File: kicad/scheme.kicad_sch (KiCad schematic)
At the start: 46 parts, among them J1 reset, Q1 G1, SW1 SW_PUSH_6mm_H4.3mm, SW2 SW_PUSH_6mm_H4.3mm, SW3 SW_PUSH_6mm_H4.3mm, SW4 btn-start, SW5 SW_PUSH_6mm_H4.3mm, U1 COM-09032-103-530, U2 ESP-12E-no_pins, U3 PCA9306, U4 AP2112K-3.3, U5 ADS1015IDGS, U6 ME6211C18M5, U7 ICM-20948

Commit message: kicad-updates
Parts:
- removed ICM-conn1: AUX-ICM-no!, Connector_PinHeader_2.54mm:PinHeader_1x04_P2.54mm_Vertical, symbol Connector:Conn_01x04_Pin
- added J2: Conn_01x04, Connector_PinSocket_2.54mm:PinSocket_1x04_P2.54mm_Vertical, symbol Connector_Generic:Conn_01x04
- added J3: poweron, Connector_PinHeader_2.54mm:PinHeader_2x01_P2.54mm_Vertical, symbol Connector:Conn_01x02_Pin
- added R16: R-100, Resistor_SMD:R_0805_2012Metric, symbol models:R-10k
- added R17: 4k7, Resistor_SMD:R_0805_2012Metric_Pad1.20x1.40mm_HandSolder, symbol Device:R_Small
- added R18: 1k, Resistor_SMD:R_0805_2012Metric_Pad1.20x1.40mm_HandSolder, symbol Device:R_Small
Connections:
- net +3.3V: now also R16.2
- net +4.2V: now also J2.1 (Pin_1), J3.1 (Pin_1); no longer TP4056-module1.3 (out+)
- net GND: now also J2.2 (Pin_2), R18.2; no longer SW4.1 (C)
- net SCL: now also J2.3 (Pin_3)
- net SDA: now also J2.4 (Pin_4)
- net bt+: now reaches BT1.+, TP4056-module1.5 (b+)
- net bt+: now also R17.1
- net at R6.1, U2.16 (GPIO15): now also SW4.1 (C)
- net at U2.2 (ADC): now also R17.2, R18.1; no longer SW4.2 (D)
- net aux-da: no longer names the net of U7.21 (AUX_DA)
- net aux_cl: no longer names the net of U7.7 (AUX_CL)
- new net: J3.2 (Pin_2), TP4056-module1.3 (out+)
- new net: R16.1, SW4.2 (D)
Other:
- note added: "ICM-version"
- moved on the sheet: C1, C10, C2, C3, C4, C5, C7, R12, R2, R3, R6, SW4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

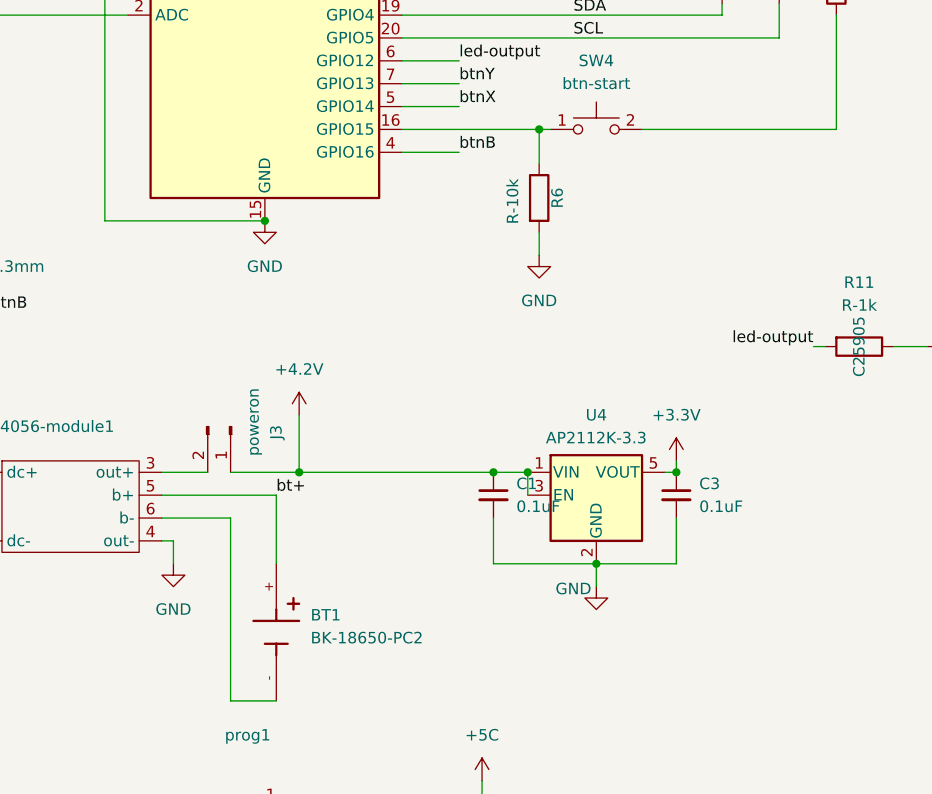
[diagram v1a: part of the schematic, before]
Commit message: changes in scheme
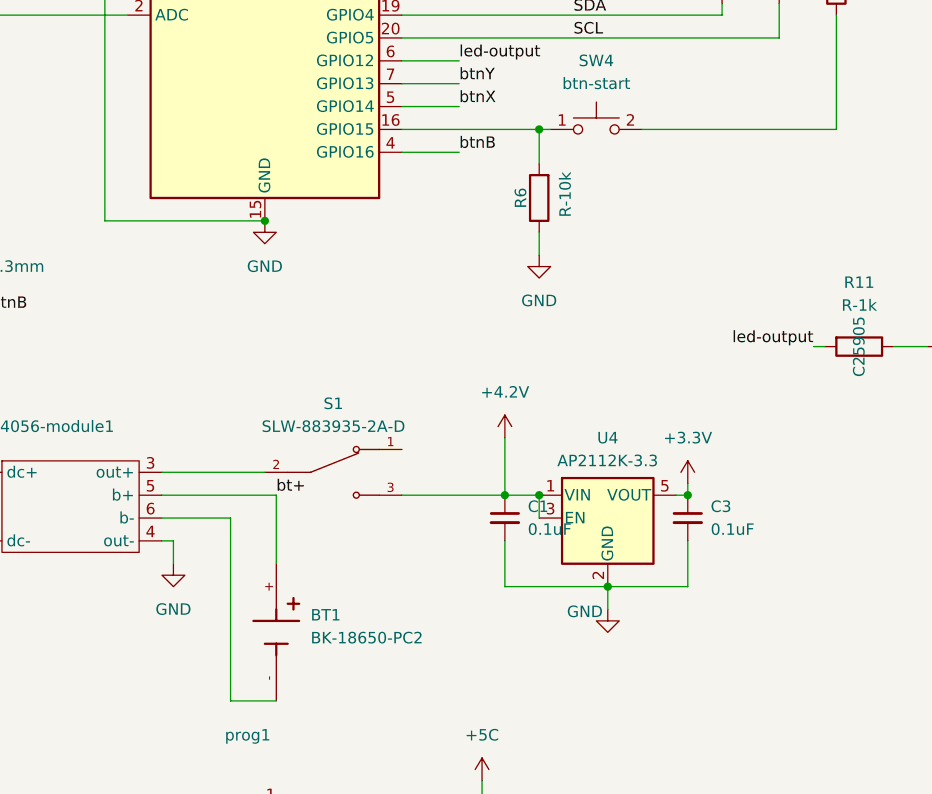
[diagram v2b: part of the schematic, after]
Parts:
- removed J3: poweron, Connector_PinHeader_2.54mm:PinHeader_2x01_P2.54mm_Vertical, symbol Connector:Conn_01x02_Pin
- added S1: SLW-883935-2A-D, module-custom-for-esp8266:SW_SLW-883935-2A-D, symbol models:SLW-883935-2A-D
- C1, C10, C2, C3, C4, C5, C8, C9: footprint Capacitor_SMD:C_0805_2012Metric -> Resistor_SMD:R_0805_2012Metric_Pad1.20x1.40mm_HandSolder
- C7: footprint Capacitor_THT:CP_Radial_D10.0mm_P3.50mm -> Resistor_SMD:R_0805_2012Metric_Pad1.20x1.40mm_HandSolder
- R11, R12, R13, R14, R15, R16, R4, R5, R6, R7, R8: footprint Resistor_SMD:R_0805_2012Metric -> Resistor_SMD:R_0805_2012Metric_Pad1.20x1.40mm_HandSolder
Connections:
- net +4.2V: now also S1.3
- net GND: now also R6.1; no longer R6.2
- net at TP4056-module1.3 (out+): now also S1.2
- net at SW4.1 (C), U2.16 (GPIO15): now also R6.2; no longer R6.1
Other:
- moved on the sheet: C1, C3, R6, U4

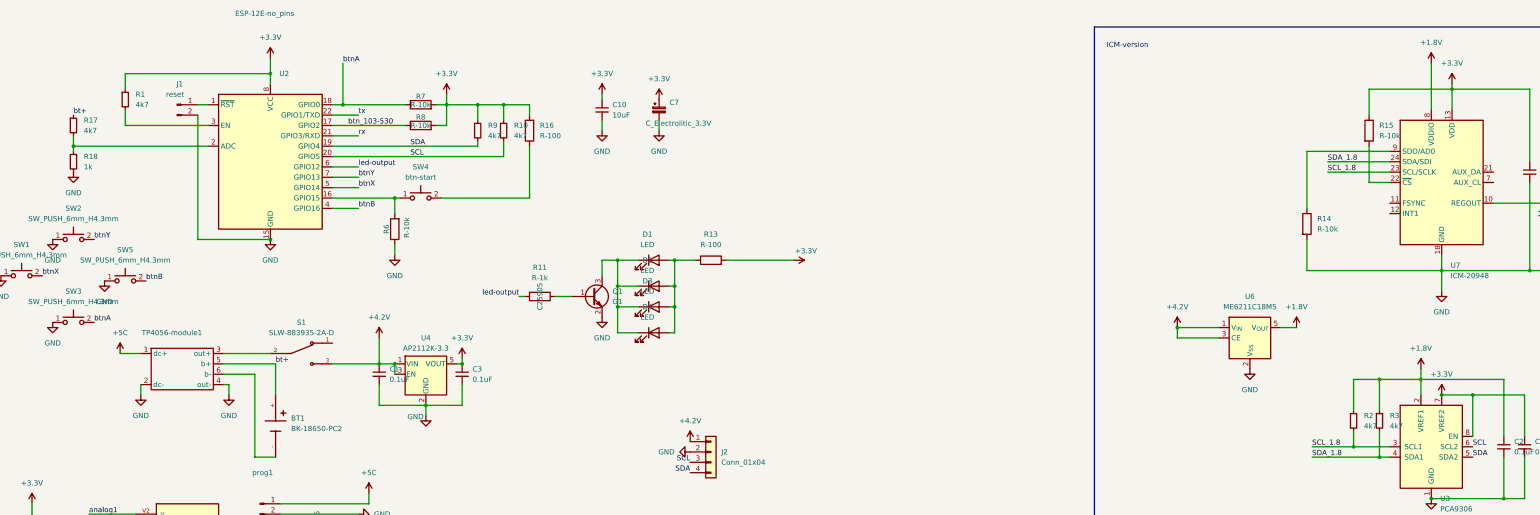
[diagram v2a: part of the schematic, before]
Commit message: added Readme
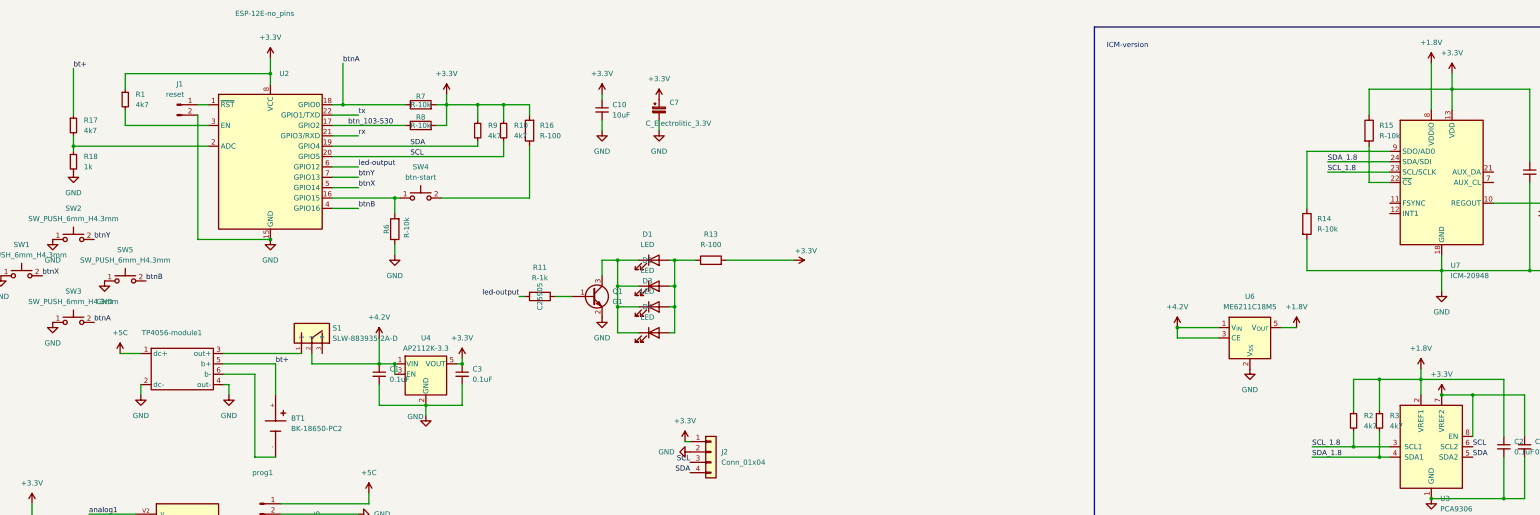
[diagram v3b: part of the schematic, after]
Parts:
- S1: footprint module-custom-for-esp8266:SW_SLW-883935-2A-D -> module-custom-for-esp8266:SW_OS102011MS2QN1_slideSwitch; symbol models:SLW-883935-2A-D -> models:OS102011MS2QN1_SlideSwitch; MP SLW-883935-2A-D -> OS102011MS2QN1
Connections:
- net +3.3V: now also J2.1 (Pin_1)
- net +4.2V: now also S1.2; no longer J2.1 (Pin_1), S1.3
- net at TP4056-module1.3 (out+): now also S1.1; no longer S1.2
